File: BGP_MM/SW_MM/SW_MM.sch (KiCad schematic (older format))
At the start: 6 parts, among them J1 Screw_Terminal_01x02, J2 Screw_Terminal_01x02, J4 Screw_Terminal_01x02, J5 Screw_Terminal_01x02, P1 CONN_01X03, SW1 SW_4PDT_x4

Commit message: MM Refactoring
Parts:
- removed SW1: SW_4PDT_x4, LIBS:NKK_DP3T, symbol SW_4PDT_x4
- added SW1: SW_4PDT, LIBS:NKK_DP3T, symbol SW_4PDT
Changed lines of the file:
@@
 LIBS:valves
 LIBS:parts
-LIBS:SW_MM_4PTT-cache
+LIBS:SW_MM-cache
 EELAYER 25 0
 EELAYER END
@@
 NBH
 $Comp
-L SW_4PDT_x4 SW1
-U 1 1 5B18C0D4
-P 6300 3650
-F 0 "SW1" H 6300 3820 50  0000 C CNN
-F 1 "SW_4PDT_x4" H 6300 3450 50  0001 C CNN
-F 2 "LIBS:NKK_DP3T" H 6300 3650 50  0001 C CNN
-F 3 "" H 6300 3650 50  0001 C CNN
-	1    6300 3650
-	1    0    0    -1
-$EndComp
-$Comp
-L SW_4PDT_x4 SW1
-U 2 1 5B18C1BA
-P 6300 4100
-F 0 "SW1" H 6300 4270 50  0000 C CNN
-F 1 "SW_4PDT_x4" H 6300 3900 50  0001 C CNN
-F 2 "LIBS:NKK_DP3T" H 6300 4100 50  0001 C CNN
-F 3 "" H 6300 4100 50  0001 C CNN
-	2    6300 4100
-	1    0    0    -1
-$EndComp
-$Comp
-L SW_4PDT_x4 SW1
-U 3 1 5B18C263
-P 4600 3650
-F 0 "SW1" H 4600 3820 50  0000 C CNN
-F 1 "SW_4PDT_x4" H 4600 3450 50  0001 C CNN
-F 2 "LIBS:NKK_DP3T" H 4600 3650 50  0001 C CNN
-F 3 "" H 4600 3650 50  0001 C CNN
-	3    4600 3650
-	1    0    0    -1
-$EndComp
-$Comp
-L SW_4PDT_x4 SW1
-U 4 1 5B18C28E
-P 4600 4100
-F 0 "SW1" H 4600 4270 50  0000 C CNN
-F 1 "SW_4PDT_x4" H 4600 3900 50  0001 C CNN
-F 2 "LIBS:NKK_DP3T" H 4600 4100 50  0001 C CNN
-F 3 "" H 4600 4100 50  0001 C CNN
-	4    4600 4100
-	1    0    0    -1
-$EndComp
-$Comp
 L CONN_01X03 P1
 U 1 1 5B18C99E
@@
 	1    0    0    -1
 $EndComp
+$Comp
+L SW_4PDT SW1
+U 3 1 5B19BB3C
+P 4600 3650
+F 0 "SW1" H 4600 3820 50  0000 C CNN
+F 1 "SW_4PDT" H 4600 3450 50  0001 C CNN
+F 2 "LIBS:NKK_DP3T" H 4600 3650 50  0001 C CNN
+F 3 "" H 4600 3650 50  0001 C CNN
+	3    4600 3650
+	1    0    0    -1
+$EndComp
+$Comp
+L SW_4PDT SW1
+U 4 1 5B19BB95
+P 4600 4100
+F 0 "SW1" H 4600 4270 50  0000 C CNN
+F 1 "SW_4PDT" H 4600 3900 50  0001 C CNN
+F 2 "LIBS:NKK_DP3T" H 4600 4100 50  0001 C CNN
+F 3 "" H 4600 4100 50  0001 C CNN
+	4    4600 4100
+	1    0    0    -1
+$EndComp
+$Comp
+L SW_4PDT SW1
+U 2 1 5B19BC05
+P 6300 4100
+F 0 "SW1" H 6300 4270 50  0000 C CNN
+F 1 "SW_4PDT" H 6300 3900 50  0001 C CNN
+F 2 "LIBS:NKK_DP3T" H 6300 4100 50  0001 C CNN
+F 3 "" H 6300 4100 50  0001 C CNN
+	2    6300 4100
+	1    0    0    -1
+$EndComp
+$Comp
+L SW_4PDT SW1
+U 1 1 5B19BE18
+P 6300 3650
+F 0 "SW1" H 6300 3820 50  0000 C CNN
+F 1 "SW_4PDT" H 6300 3450 50  0001 C CNN
+F 2 "LIBS:NKK_DP3T" H 6300 3650 50  0001 C CNN
+F 3 "" H 6300 3650 50  0001 C CNN
+	1    6300 3650
+	1    0    0    -1
+$EndComp

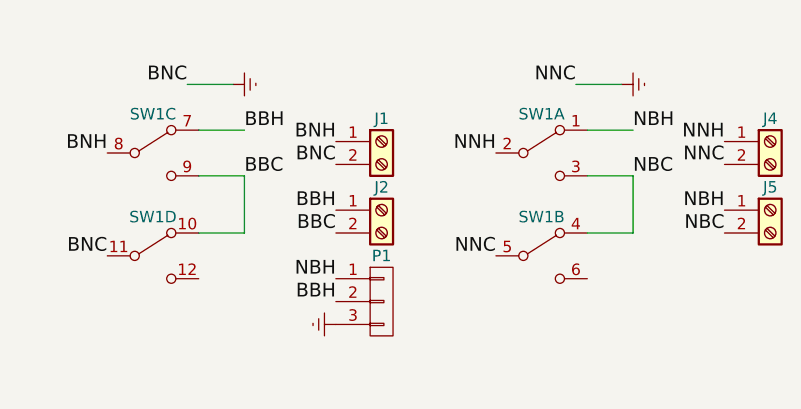
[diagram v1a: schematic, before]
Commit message: MM Refactoring
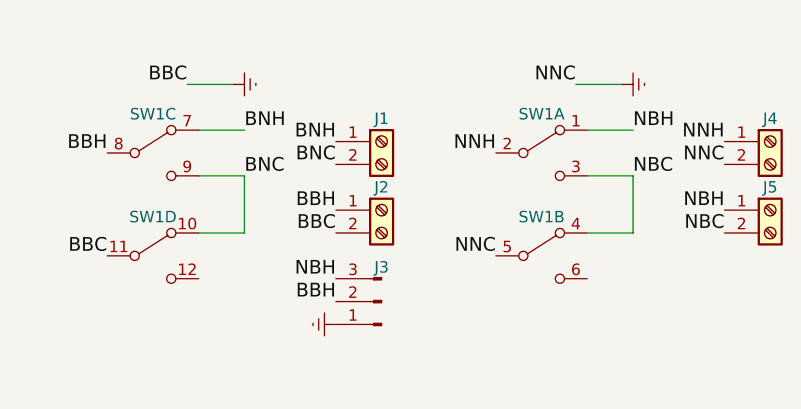
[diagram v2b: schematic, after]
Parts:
- removed P1: CONN_01X03, Connectors_JST:JST_PH_B3B-PH-K_03x2.00mm_Straight, symbol CONN_01X03
- added J3: Conn_01x03_Male, Pin_Headers:Pin_Header_Straight_1x03_Pitch2.54mm, symbol Conn_01x03_Male
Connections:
- net BBH: now also SW1.8 (B), J3.2 (Pin_2); no longer SW1.7 (A)
- net BNH: now also SW1.7 (A); no longer SW1.8 (B)
- net Earth: now also J2.2 (Pin_2), J3.1 (Pin_1); no longer J1.2 (Pin_2)
- net NBH: now also J3.3 (Pin_3)
- net BBC renamed BNC
- net BNC: now also J1.2 (Pin_2); no longer J2.2 (Pin_2)
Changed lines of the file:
@@
 $EndDescr
 Text Label 5000 3550 0    60   ~ 0
+BNH
+Text Label 4400 3650 2    60   ~ 0
 BBH
-Text Label 4400 3650 2    60   ~ 0
-BNH
 Wire Wire Line
 	5000 4000 5000 3750
 Text Label 5000 3750 0    60   ~ 0
+BNC
+Text Label 4400 4100 2    60   ~ 0
 BBC
-Text Label 4400 4100 2    60   ~ 0
-BNC
 Text Label 5400 3900 2    60   ~ 0
 BBH
@@
 	4950 3350 4750 3350
 Text Label 4750 3350 2    60   ~ 0
-BNC
+BBC
 Text Label 5400 4300 2    60   ~ 0
 BBH
@@
 NBH
 $Comp
-L CONN_01X03 P1
-U 1 1 5B18C99E
-P 5600 4300
-F 0 "P1" H 5600 4500 50  0000 C CNN
-F 1 "CONN_01X03" V 5700 4300 50  0001 C CNN
-F 2 "Connectors_JST:JST_PH_B3B-PH-K_03x2.00mm_Straight" H 5600 4300 50  0001 C CNN
-F 3 "" H 5600 4300 50  0000 C CNN
-	1    5600 4300
-	1    0    0    -1
-$EndComp
-$Comp
 L SW_4PDT SW1
 U 3 1 5B19BB3C
@@
 	1    0    0    -1
 $EndComp
+$Comp
+L Conn_01x03_Male J3
+U 1 1 5B1B17BF
+P 5600 4300
+F 0 "J3" H 5600 4150 50  0000 C CNN
+F 1 "Conn_01x03_Male" H 5600 4100 50  0001 C CNN
+F 2 "Pin_Headers:Pin_Header_Straight_1x03_Pitch2.54mm" H 5600 4300 50  0001 C CNN
+F 3 "" H 5600 4300 50  0001 C CNN
+	1    5600 4300
+	-1   0    0    1
+$EndComp
 $EndSCHEMATC
